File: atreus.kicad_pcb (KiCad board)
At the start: 2 copper layers, 232 x 90 mm, 85 parts

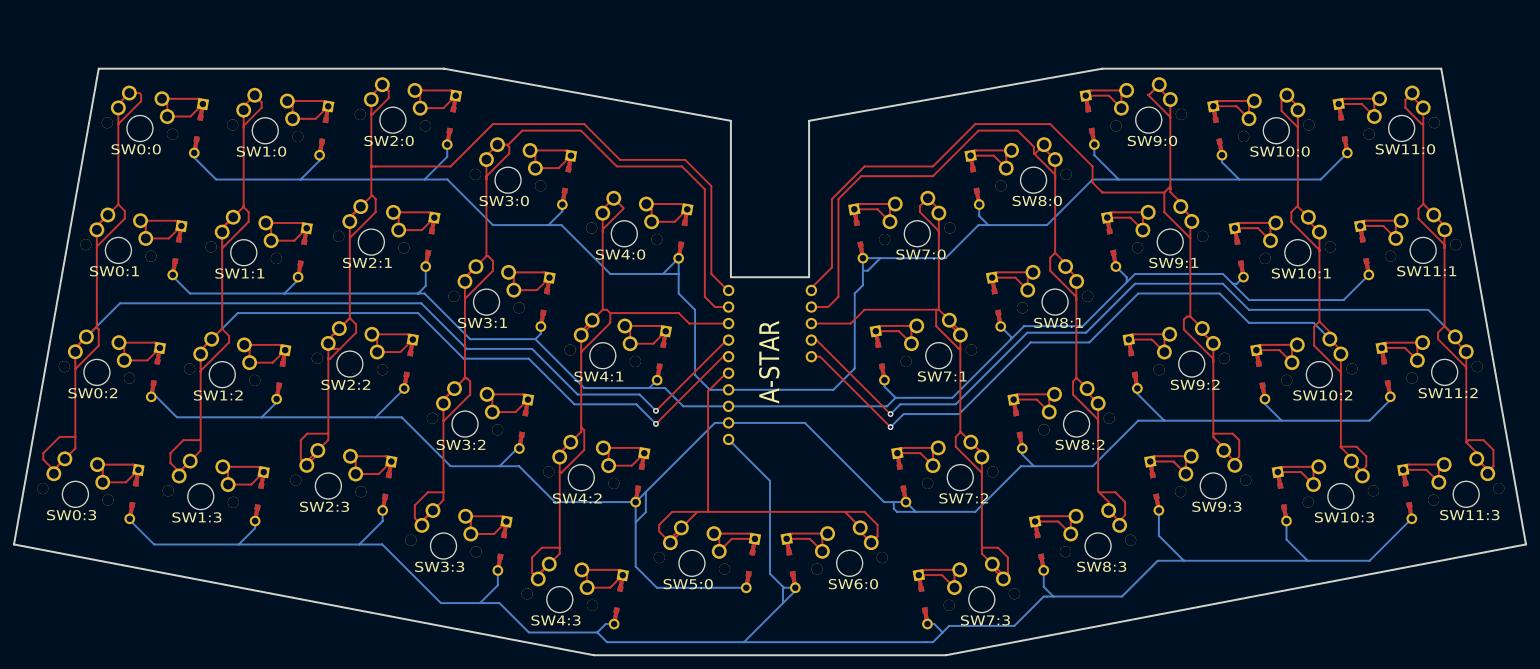
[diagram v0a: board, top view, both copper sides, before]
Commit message: changes
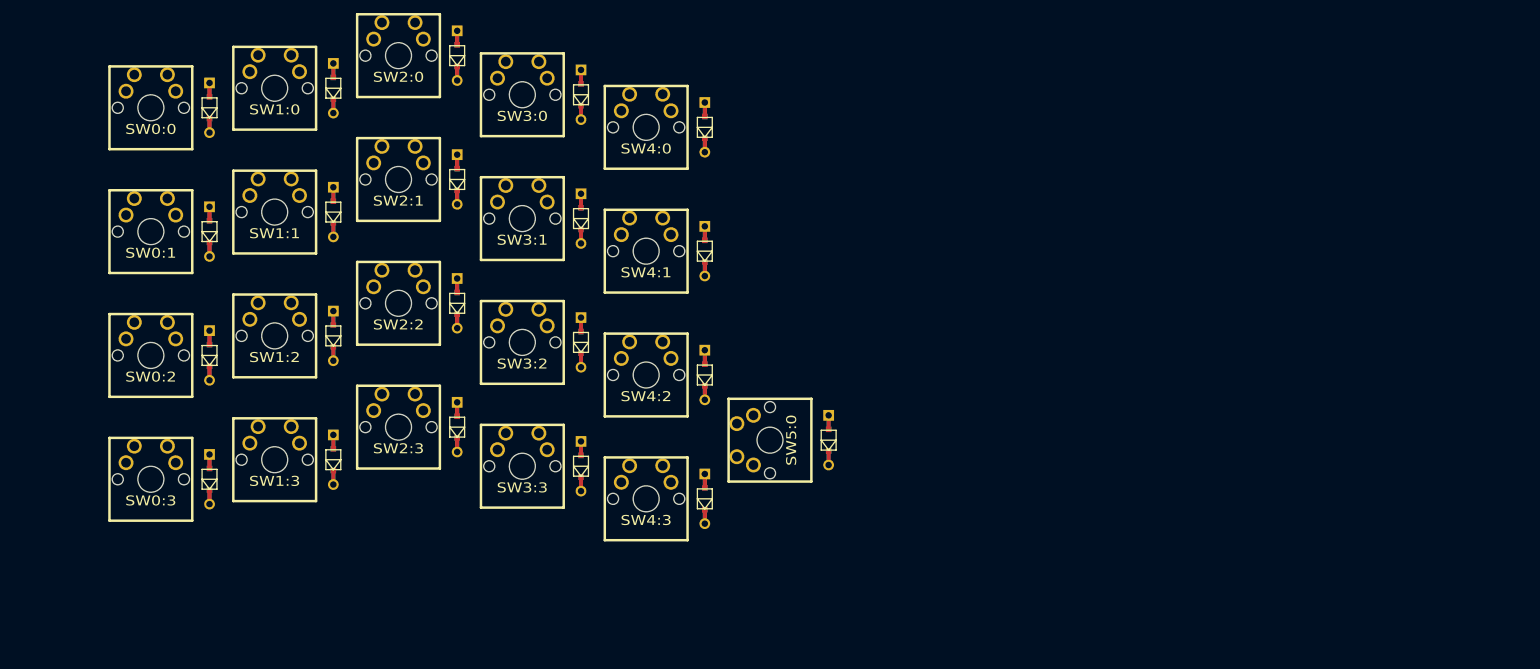
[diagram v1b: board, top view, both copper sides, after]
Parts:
- removed ?: A-STAR, A_STAR
- removed the D2:2 at (46.3, 31.2)
- removed the D2:2 at (81.8, 48.6)
- removed the D2:2 at (78.5, 67.3)
- removed the D2:2 at (75.2, 86.0)
- removed the D2:2 at (102.8, 39.1)
- removed the D2:2 at (99.5, 57.8)
- removed the D2:2 at (96.2, 76.5)
- removed the D2:2 at (92.9, 95.2)
- removed the D2:2 at (120.6, 47.3)
- removed the D2:2 at (117.3, 66.0)
- removed the D2:2 at (114.0, 84.8)
- removed the D2:2 at (43.0, 49.9)
- removed the D2:2 at (110.7, 103.5)
- removed the D2:2 at (131.0, 97.9)
- removed the D2:2 at (137.2, 97.9)
- removed the D2:2 at (147.6, 47.3)
- removed the D2:2 at (150.9, 66.0)
- removed the D2:2 at (154.2, 84.7)
- removed the D2:2 at (157.5, 103.5)
- removed the D2:2 at (165.4, 39.1)
- removed the D2:2 at (168.7, 57.8)
- removed the D2:2 at (172.0, 76.5)
- removed the D2:2 at (39.7, 68.6)
- removed the D2:2 at (175.3, 95.2)
- removed the D2:2 at (183.1, 29.9)
- removed the D2:2 at (186.4, 48.6)
- removed the D2:2 at (189.7, 67.3)
- removed the D2:2 at (193.0, 86.0)
- removed the D2:2 at (202.7, 31.5)
- removed the D2:2 at (206.0, 50.2)
- removed the D2:2 at (209.3, 68.9)
- removed the D2:2 at (212.6, 87.7)
- removed the D2:2 at (221.9, 31.2)
- removed the D2:2 at (36.4, 87.3)
- removed the D2:2 at (225.2, 49.9)
- removed the D2:2 at (228.5, 68.6)
- removed the D2:2 at (231.8, 87.3)
- removed the D2:2 at (65.6, 31.5)
- removed the D2:2 at (62.3, 50.2)
- removed the D2:2 at (59.0, 68.9)
- removed the D2:2 at (55.7, 87.7)
- removed the D2:2 at (85.1, 29.9)
- removed SW10:0, SW10:1, SW10:2, SW10:3, SW11:0, SW11:1, SW11:2, SW11:3, SW6:0, SW7:0, SW7:1, SW7:2, SW7:3, SW8:0, SW8:1, SW8:2, SW8:3, SW9:0, SW9:1, SW9:2, SW9:3: , MX_FLIP
- added D2:2: , DIODE, F.Cu at (48.0, 28.0)
- added D2:2: , DIODE, F.Cu at (86.0, 39.0)
- added D2:2: , DIODE, F.Cu at (86.0, 58.0)
- added D2:2: , DIODE, F.Cu at (86.0, 77.0)
- added D2:2: , DIODE, F.Cu at (105.0, 26.0)
- added D2:2: , DIODE, F.Cu at (105.0, 45.0)
- added D2:2: , DIODE, F.Cu at (105.0, 64.0)
- added D2:2: , DIODE, F.Cu at (105.0, 83.0)
- added D2:2: , DIODE, F.Cu at (124.0, 31.0)
- added D2:2: , DIODE, F.Cu at (124.0, 50.0)
- added D2:2: , DIODE, F.Cu at (124.0, 69.0)
- added D2:2: , DIODE, F.Cu at (48.0, 47.0)
- added D2:2: , DIODE, F.Cu at (124.0, 88.0)
- added D2:2: , DIODE, F.Cu at (143.0, 79.0)
- added D2:2: , DIODE, F.Cu at (48.0, 66.0)
- added D2:2: , DIODE, F.Cu at (48.0, 85.0)
- added D2:2: , DIODE, F.Cu at (67.0, 25.0)
- added D2:2: , DIODE, F.Cu at (67.0, 44.0)
- added D2:2: , DIODE, F.Cu at (67.0, 63.0)
- added D2:2: , DIODE, F.Cu at (67.0, 82.0)
- added D2:2: , DIODE, F.Cu at (86.0, 20.0)
- moved SW5:0 22.4 mm to (134.0, 79.0), turned to 90 degrees
- moved SW4:3 20.4 mm to (115.0, 88.0), turned to 0 degrees
- moved SW4:2 18.6 mm to (115.0, 69.0), turned to 0 degrees
- moved SW4:1 17.4 mm to (115.0, 50.0), turned to 0 degrees
- moved SW3:3 17.2 mm to (96.0, 83.0), turned to 0 degrees
- moved SW4:0 16.7 mm to (115.0, 31.0), turned to 0 degrees
- moved SW3:2 15.3 mm to (96.0, 64.0), turned to 0 degrees
- moved SW2:3 14.1 mm to (77.0, 77.0), turned to 0 degrees
- moved SW3:1 13.9 mm to (96.0, 45.0), turned to 0 degrees
- moved SW3:0 13.3 mm to (96.0, 26.0), turned to 0 degrees
- moved SW1:3 12.7 mm to (58.0, 82.0), turned to 0 degrees
- moved SW2:2 11.9 mm to (77.0, 58.0), turned to 0 degrees
- moved SW0:3 11.8 mm to (39.0, 85.0), turned to 0 degrees
- moved SW2:1 10.5 mm to (77.0, 39.0), turned to 0 degrees
- moved SW1:2 10.0 mm to (58.0, 63.0), turned to 0 degrees
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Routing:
- net N-row-3: track 299.5 -> 0.00 mm
- net N-row-2: track 281.8 -> 0.00 mm
- net N-row-0: track 264.8 -> 0.00 mm
- net N-row-1: track 226.9 -> 0.00 mm
- net N-col-0: track 218.7 -> 0.00 mm, vias 1 -> 0
- net N-col-10: track 211.5 -> 0.00 mm, vias 1 -> 0
- net N-col-1: track 197.0 -> 0.00 mm, vias 1 -> 0
- net N-col-9: track 193.0 -> 0.00 mm, vias 1 -> 0
- net N-col-2: track 189.2 -> 0.00 mm
- net N-col-8: track 176.2 -> 0.00 mm
- net N-col-3: track 162.6 -> 0.00 mm
- net N-col-7: track 153.6 -> 0.00 mm
- net N-col-6: track 124.5 -> 0.00 mm
- net N-col-4: track 124.1 -> 0.00 mm
- net N-col-5: track 80.4 -> 0.00 mm
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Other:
- board outline removed
